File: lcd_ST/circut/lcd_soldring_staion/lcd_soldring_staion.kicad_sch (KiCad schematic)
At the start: 2 parts, among them U1 PIC16F876-XXISP, U2 L7805

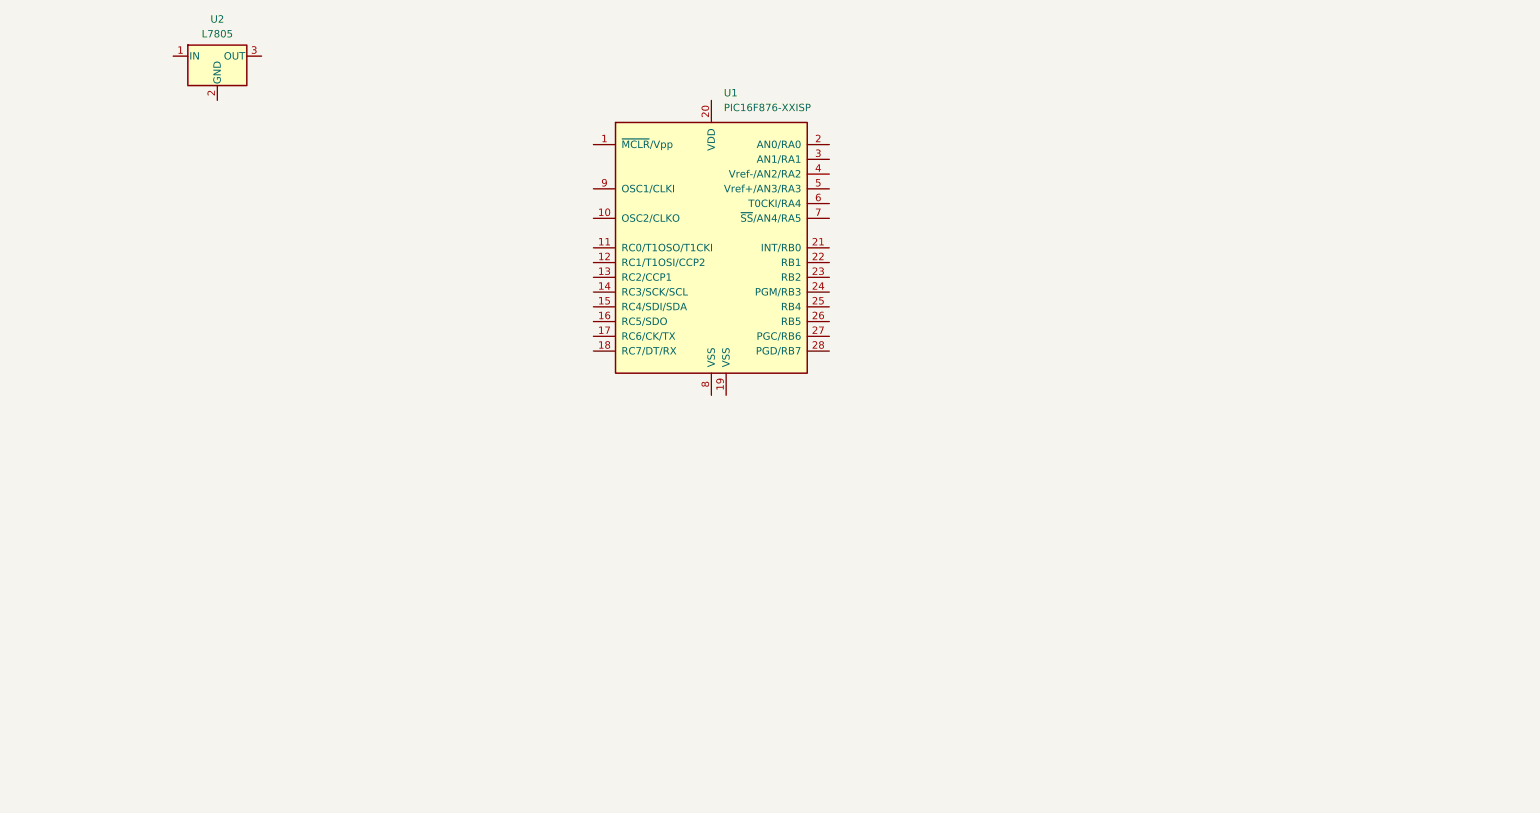
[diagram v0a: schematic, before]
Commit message: Update lcd_soldring_staion.kicad_sch
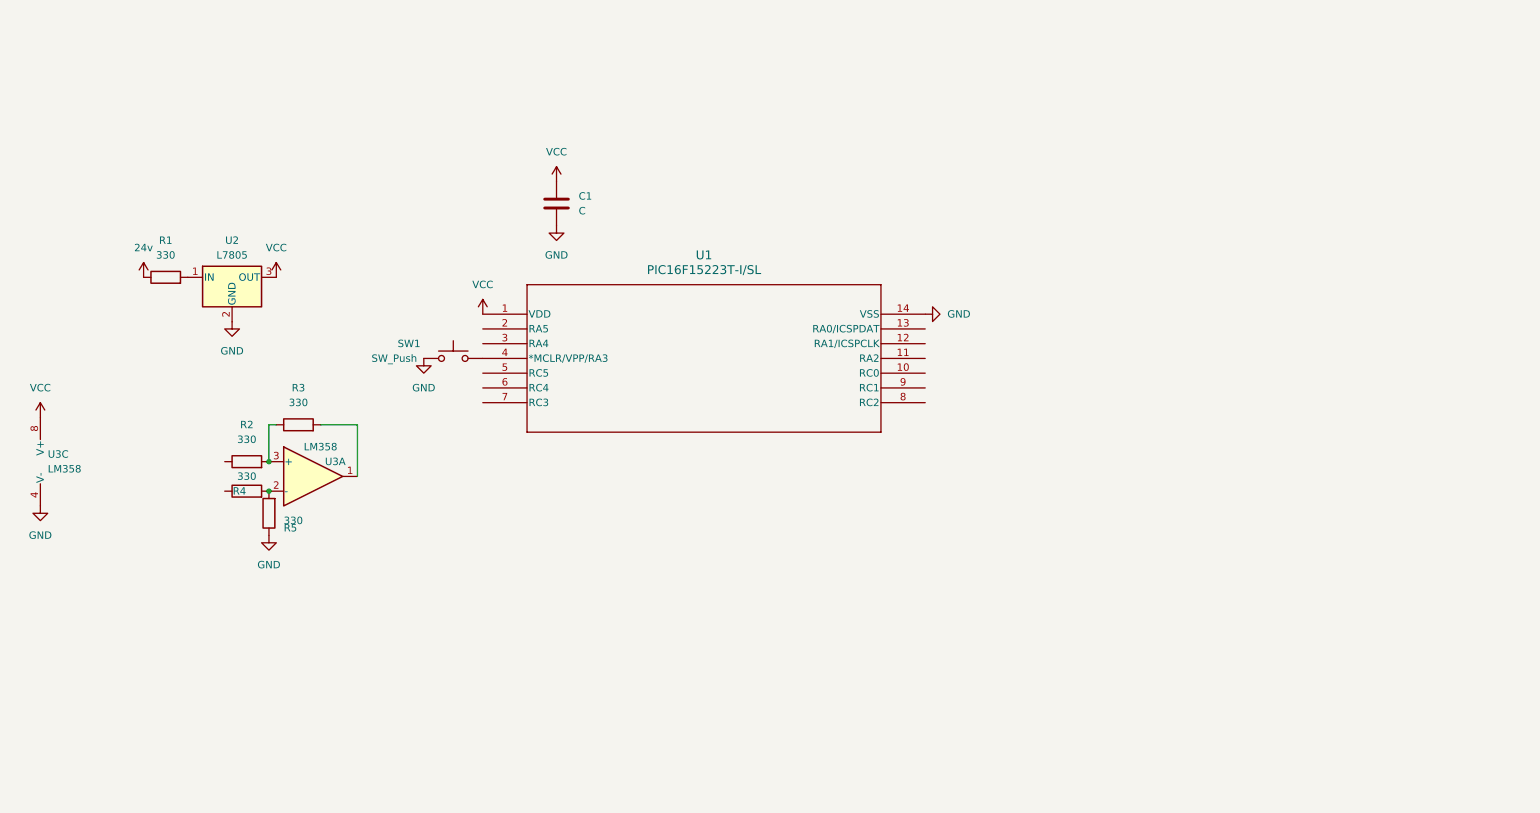
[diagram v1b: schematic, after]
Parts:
- removed U1: PIC16F876-XXISP, Package_DIP:DIP-28_W7.62mm_LongPads, symbol MCU_Microchip_PIC16:PIC16F876-XXISP
- added C1: C, symbol Device:C
- added R1, R2, R3, R4, R5: 330, symbol Device:R
- added SW1: SW_Push, symbol Switch:SW_Push
- added U1: PIC16F15223T-I/SL, SOIC14_SL_MCH, symbol pic16f15223:PIC16F15223T-I_SL
- added U3: LM358, symbol Amplifier_Operational:LM358
- U2: footprint Package_TO_SOT_SMD:TO-252-3_TabPin2 -> (none)
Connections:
- net at U2.1 (IN): now also R1.2
- net GND: now reaches U2.2 (GND)
- net GND: now also C1.2, R5.1, SW1.1, U1.14 (VSS), U3.4 (V-)
- net VCC: now reaches U2.3 (OUT)
- net VCC: now also C1.1, U1.1 (VDD), U3.8 (V+)
- new net: SW1.2, U1.4 (*MCLR/VPP/RA3)
- new net: R4.2, R5.2, U3.2 (-)
- new net: R3.2, U3.1
- new net: R2.2, R3.1, U3.3 (+)
- new net 24v: R1.1

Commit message: Update lcd_soldring_staion.kicad_sch
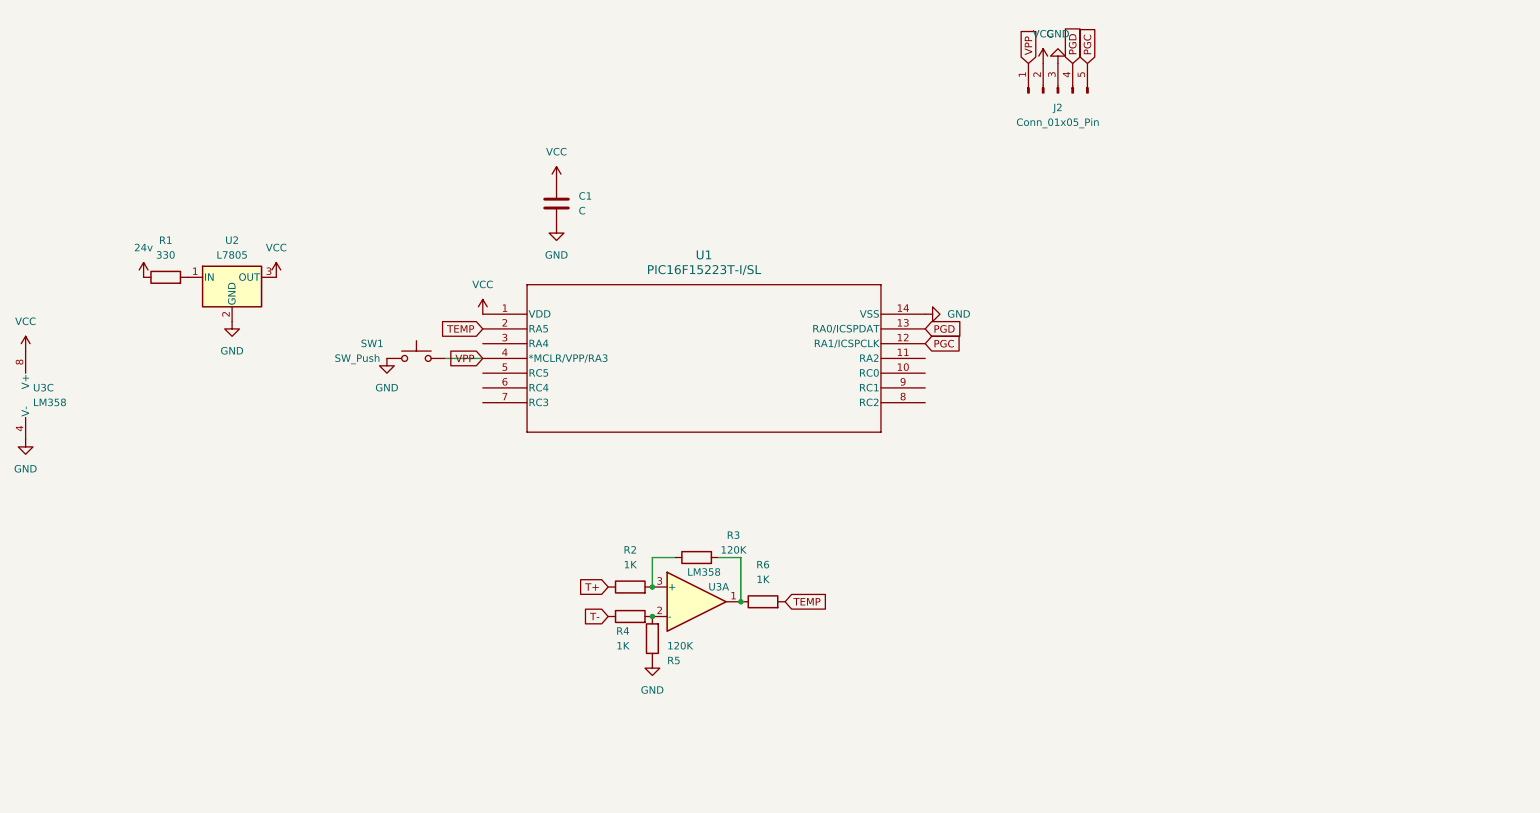
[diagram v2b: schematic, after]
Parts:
- added J2: Conn_01x05_Pin, symbol Connector:Conn_01x05_Pin
- added R6: 1K, symbol Device:R
- R2, R4: value 330 -> 1K
- R3, R5: value 330 -> 120K
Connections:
- net GND: now also J2.3 (Pin_3)
- net VCC: now also J2.2 (Pin_2)
- net VPP: now reaches SW1.2, U1.4 (*MCLR/VPP/RA3)
- net VPP: now also J2.1 (Pin_1)
- net T-: now reaches R4.1
- net PGC: now reaches U1.12 (RA1/ICSPCLK)
- net PGC: now also J2.5 (Pin_5)
- net PGD: now reaches U1.13 (RA0/ICSPDAT)
- net PGD: now also J2.4 (Pin_4)
- net TEMP: now reaches U1.2 (RA5)
- net TEMP: now also R6.2
- net at R3.2, U3.1: now also R6.1
- net T+: now reaches R2.1
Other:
- moved on the sheet: R2, R3, R4, R5, SW1, U3A, U3C

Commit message: Update lcd_soldring_staion.kicad_sch
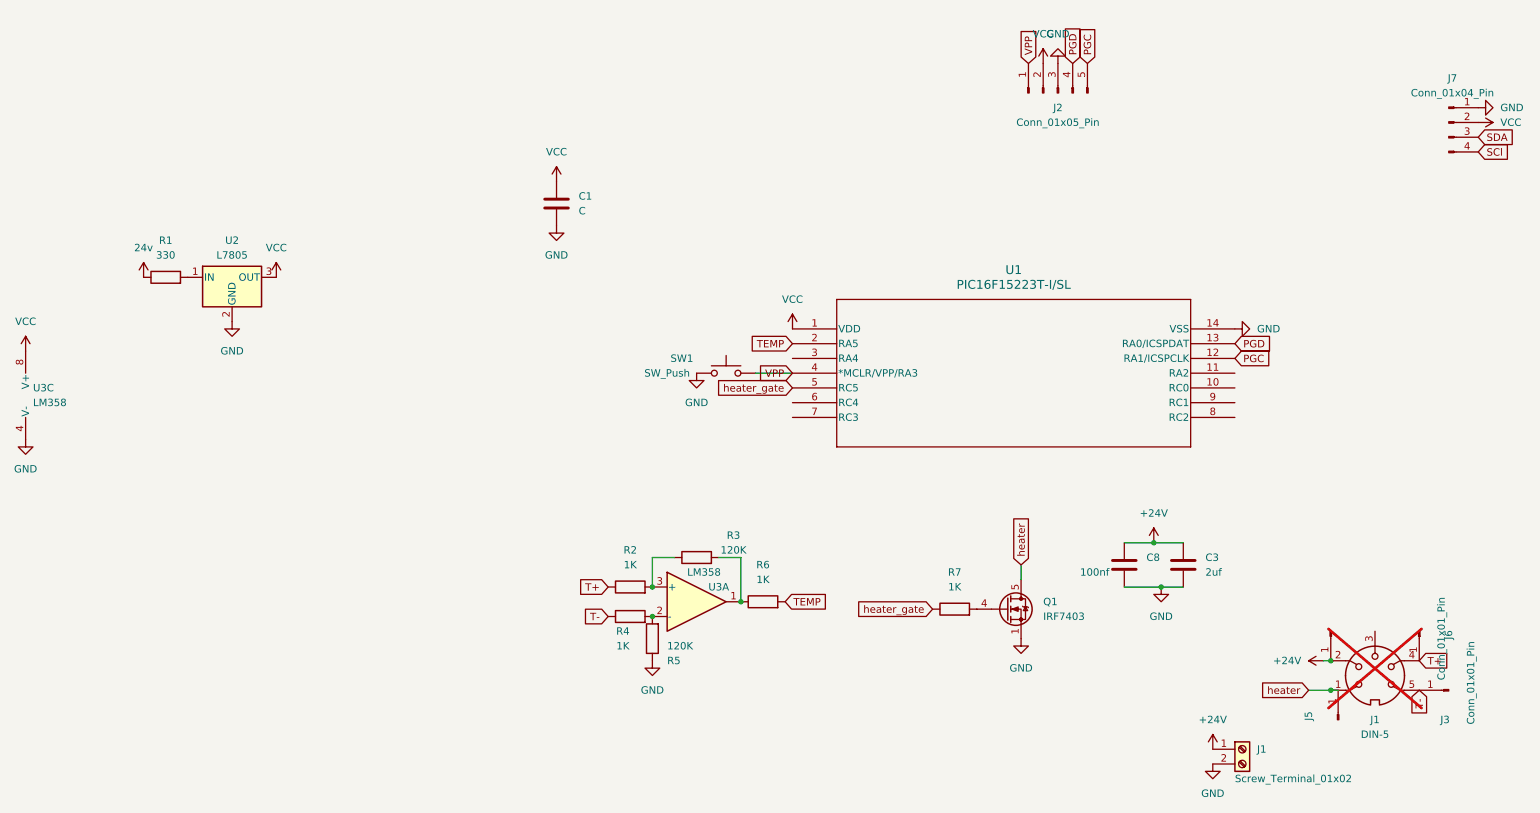
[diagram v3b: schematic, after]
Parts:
- added C3: 2uf, Capacitor_SMD:C_1206_3216Metric_Pad1.33x1.80mm_HandSolder, symbol Device:C
- added C8: 100nf, Capacitor_SMD:C_1206_3216Metric_Pad1.33x1.80mm_HandSolder, symbol Device:C
- added J1: Screw_Terminal_01x02, TerminalBlock:TerminalBlock_MaiXu_MX126-5.0-02P_1x02_P5.00mm, symbol Connector:Screw_Terminal_01x02
- added J1: DIN-5, symbol Connector:DIN-5
- added J3: Conn_01x01_Pin, Connector_JST:JST_XH_B1B-XH-AM_1x01_P2.50mm_Vertical, symbol Connector:Conn_01x01_Pin
- added J4, J5, J6: Conn_01x01_Pin, Connector_PinHeader_2.54mm:PinHeader_1x01_P2.54mm_Horizontal, symbol Connector:Conn_01x01_Pin
- added J7: Conn_01x04_Pin, symbol Connector:Conn_01x04_Pin
- added Q1: IRF7403, Package_TO_SOT_SMD:Infineon_PG-HSOF-8-3_ThermalVias, symbol Transistor_FET:IRF7403
- added R7: 1K, symbol Device:R
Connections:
- net GND: now also C3.2, C8.2, J1.2 (Pin_2), J7.1 (Pin_1), Q1.1 (S), Q1.2 (S), Q1.3 (S)
- net T+: now also J1.4, J6.1 (Pin_1)
- net T-: now also J1.5, J3.1 (Pin_1)
- net VCC: now also J7.2 (Pin_2)
- net heater_gate: now reaches U1.5 (RC5)
- net heater_gate: now also R7.1
- new net: Q1.4 (G), R7.2
- new net +24V: C3.1, C8.1, J1.1 (Pin_1), J1.2, J4.1 (Pin_1)
- new net SCl: J7.4 (Pin_4)
- new net SDA: J7.3 (Pin_3)
- new net heater: J1.1, J5.1 (Pin_1), Q1.5 (D), Q1.6 (D), Q1.7 (D), Q1.8 (D)
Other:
- moved on the sheet: SW1, U1

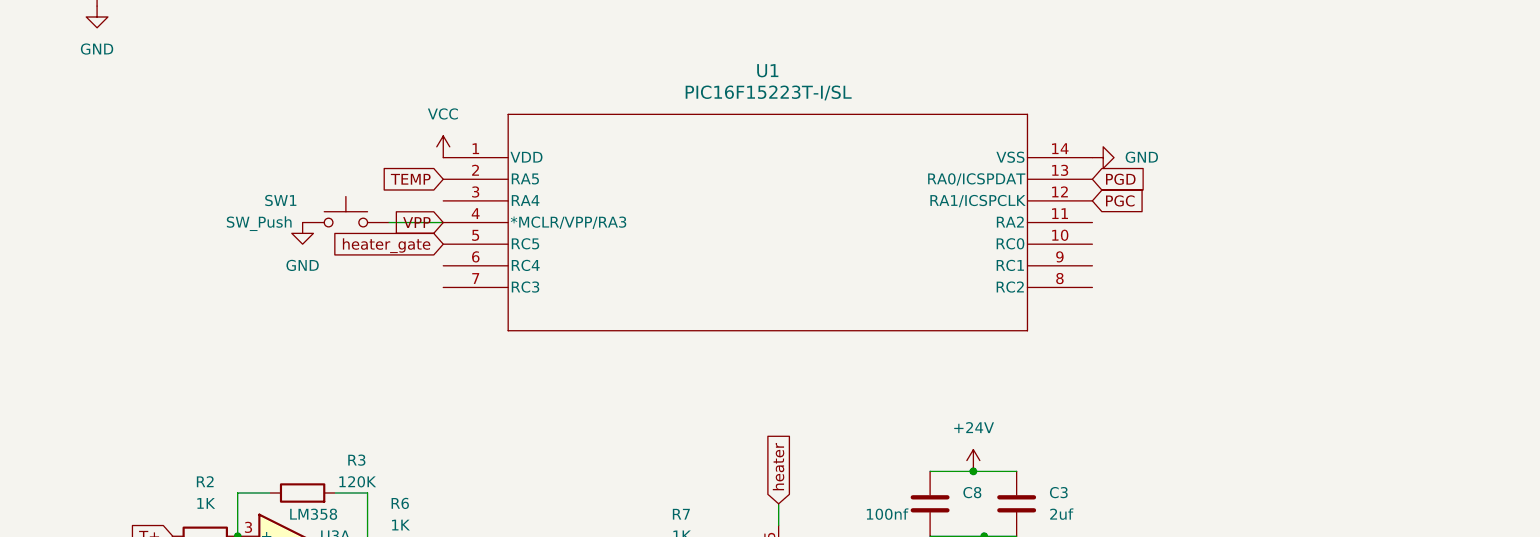
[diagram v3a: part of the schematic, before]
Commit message: Update lcd_soldring_staion.kicad_sch
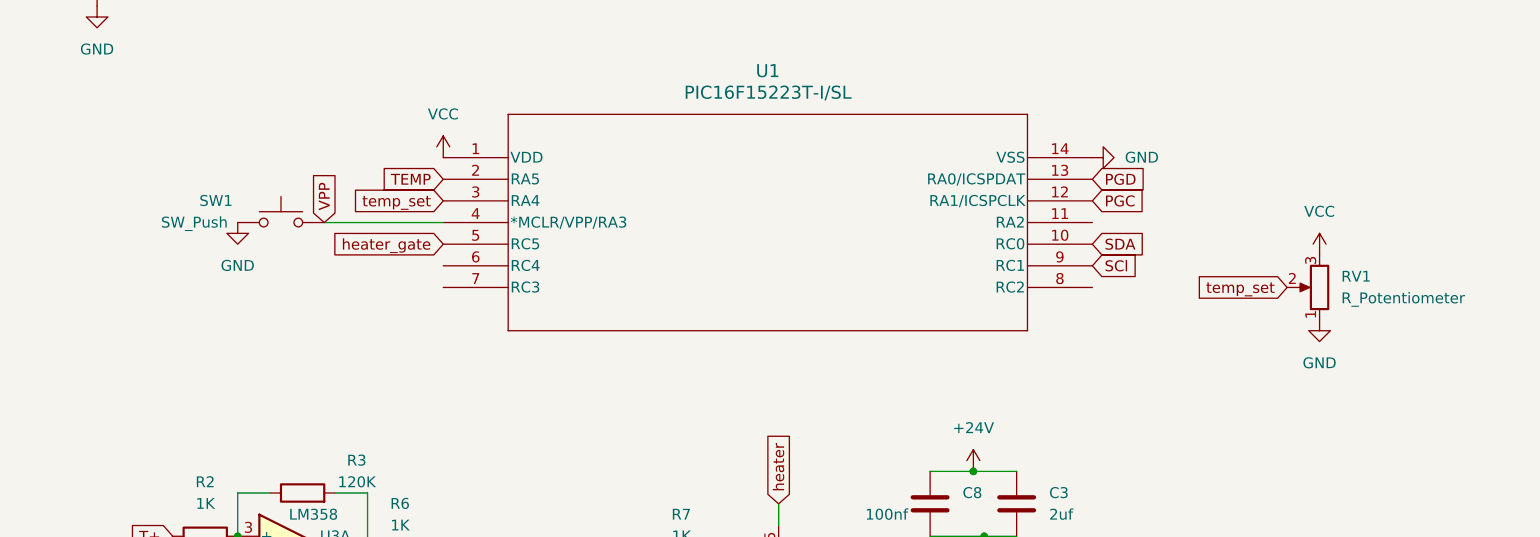
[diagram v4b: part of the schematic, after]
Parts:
- added RV1: R_Potentiometer, symbol Device:R_Potentiometer
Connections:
- net GND: now also RV1.1
- net SCl: now also U1.9 (RC1)
- net SDA: now also U1.10 (RC0)
- net VCC: now also RV1.3
- net temp_set: now reaches U1.3 (RA4)
- net temp_set: now also RV1.2
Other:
- moved on the sheet: SW1
